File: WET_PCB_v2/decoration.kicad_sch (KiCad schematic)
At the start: 12 parts, among them J12 Fuse holder or smth to hold t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, J13 Fuse holder or smth to hold t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, J14 Fuse holder or smth to hold t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, J15 Fuse holder or smth to hold t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

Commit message: redid part of layout inverter
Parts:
- D19, D20, D21, D22: footprint LED_SMD:LED_1W_3W_R8 -> LED_SMD:LED_PLCC-2_3.4x3.0mm_AK
- R29, R30, R31, R32: footprint Resistor_THT:R_Axial_DIN0207_L6.3mm_D2.5mm_P7.62mm_Horizontal -> Resistor_SMD:R_0805_2012Metric_Pad1.20x1.40mm_HandSolder
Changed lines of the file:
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@@
 			)
 		)
-		(property "Footprint" "Resistor_THT:R_Axial_DIN0207_L6.3mm_D2.5mm_P7.62mm_Horizontal"
+		(property "Footprint" "Resistor_SMD:R_0805_2012Metric_Pad1.20x1.40mm_HandSolder"
 			(at 119.38 89.408 90)
 			(hide yes)
@@
 			)
 		)
-		(property "Footprint" "Resistor_THT:R_Axial_DIN0207_L6.3mm_D2.5mm_P7.62mm_Horizontal"
+		(property "Footprint" "Resistor_SMD:R_0805_2012Metric_Pad1.20x1.40mm_HandSolder"
 			(at 119.38 110.998 90)
 			(hide yes)
@@
 			)
 		)
-		(property "Footprint" "Resistor_THT:R_Axial_DIN0207_L6.3mm_D2.5mm_P7.62mm_Horizontal"
+		(property "Footprint" "Resistor_SMD:R_0805_2012Metric_Pad1.20x1.40mm_HandSolder"
 			(at 119.38 79.248 90)
 			(hide yes)
@@
 			)
 		)
-		(property "Footprint" "LED_SMD:LED_1W_3W_R8"
+		(property "Footprint" "LED_SMD:LED_PLCC-2_3.4x3.0mm_AK"
 			(at 111.76 109.22 0)
 			(hide yes)
@@
 			)
 		)
-		(property "Footprint" "LED_SMD:LED_1W_3W_R8"
+		(property "Footprint" "LED_SMD:LED_PLCC-2_3.4x3.0mm_AK"
 			(at 111.76 77.47 0)
 			(hide yes)
@@
 			)
 		)
-		(property "Footprint" "LED_SMD:LED_1W_3W_R8"
+		(property "Footprint" "LED_SMD:LED_PLCC-2_3.4x3.0mm_AK"
 			(at 111.76 87.63 0)
 			(hide yes)
@@
 			)
 		)
-		(property "Footprint" "LED_SMD:LED_1W_3W_R8"
+		(property "Footprint" "LED_SMD:LED_PLCC-2_3.4x3.0mm_AK"
 			(at 111.76 97.79 0)
 			(hide yes)
@@
 			)
 		)
-		(property "Footprint" "Resistor_THT:R_Axial_DIN0207_L6.3mm_D2.5mm_P7.62mm_Horizontal"
+		(property "Footprint" "Resistor_SMD:R_0805_2012Metric_Pad1.20x1.40mm_HandSolder"
 			(at 119.38 99.568 90)
 			(hide yes)

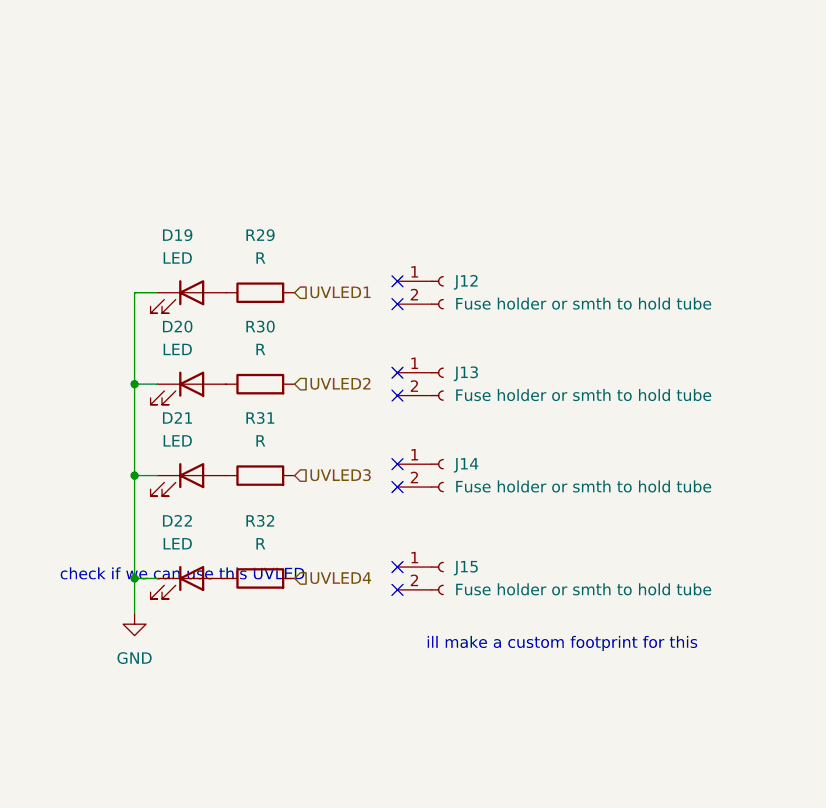
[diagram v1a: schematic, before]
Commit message: before i prob fuck up everything bc clearance
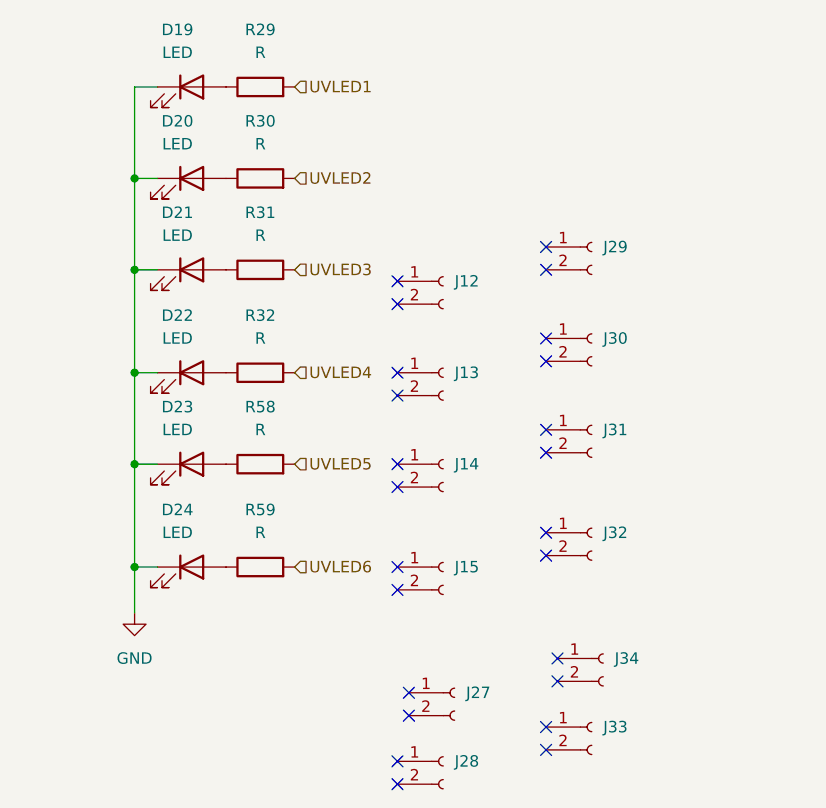
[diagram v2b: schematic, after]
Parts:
- added D23, D24: LED, LED_SMD:LED_PLCC-2_3.4x3.0mm_AK, symbol Device:LED
- added J27, J28, J29, J30, J31, J32, J33, J34: Fuse holder or smth to hold tube, TestPoint:TestPoint_Loop_D2.60mm_Drill0.9mm_Beaded, symbol Connector:Conn_01x02_Socket
- added R58, R59: R, Resistor_SMD:R_0805_2012Metric_Pad1.20x1.40mm_HandSolder, symbol Device:R
- J12, J13, J14, J15: footprint (none) -> TestPoint:TestPoint_Loop_D2.60mm_Drill0.9mm_Beaded
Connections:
- net GND: now also D23.1 (K), D24.1 (K)
- new net: D24.2 (A), R59.1
- new net: D23.2 (A), R58.1
- new net UVLED5: R58.2
- new net UVLED6: R59.2
- no-connect marks 8 -> 24
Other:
- note removed: "check if we can use this UVLED"
- note removed: "ill make a custom footprint for this"
- moved on the sheet: D19, D20, D21, D22, R29, R30, R31, R32
